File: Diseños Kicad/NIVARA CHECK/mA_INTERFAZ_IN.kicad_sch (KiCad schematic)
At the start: 1 part

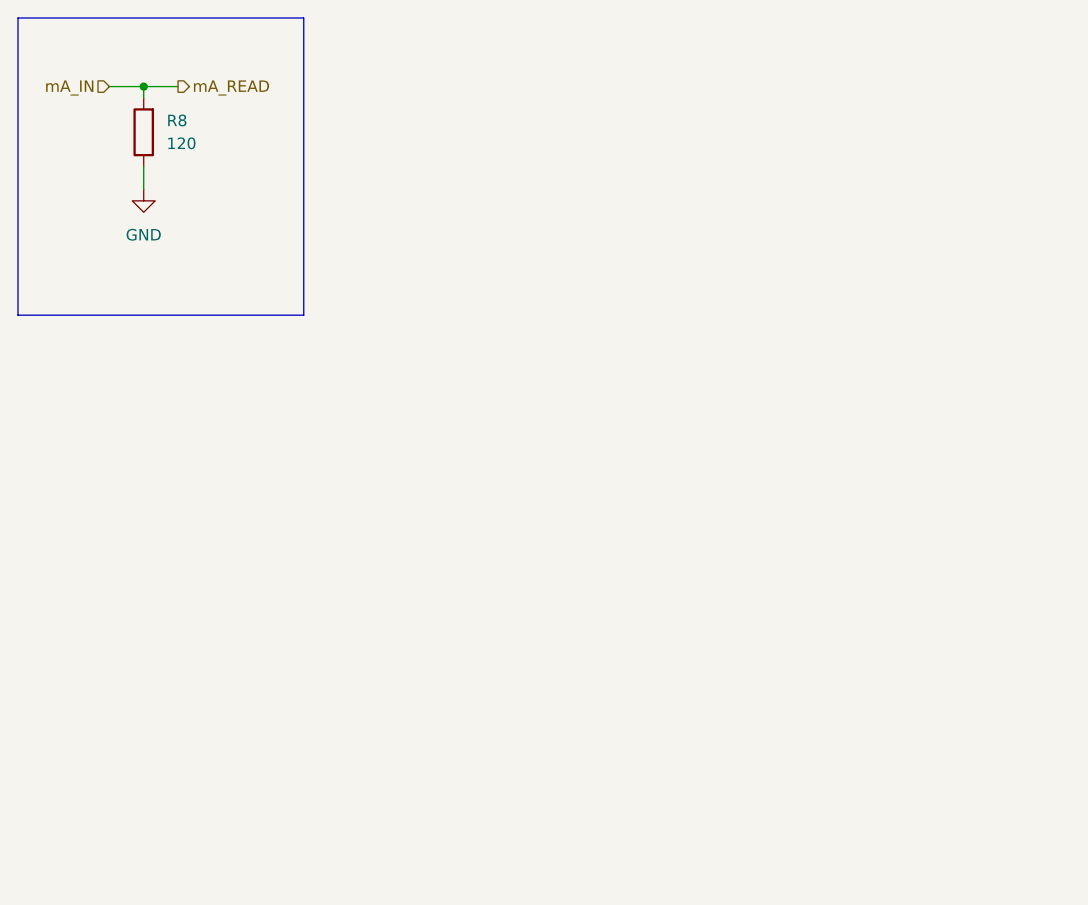
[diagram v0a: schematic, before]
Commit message: ACTUALIZACION HECHA
PCB SUPUESTA
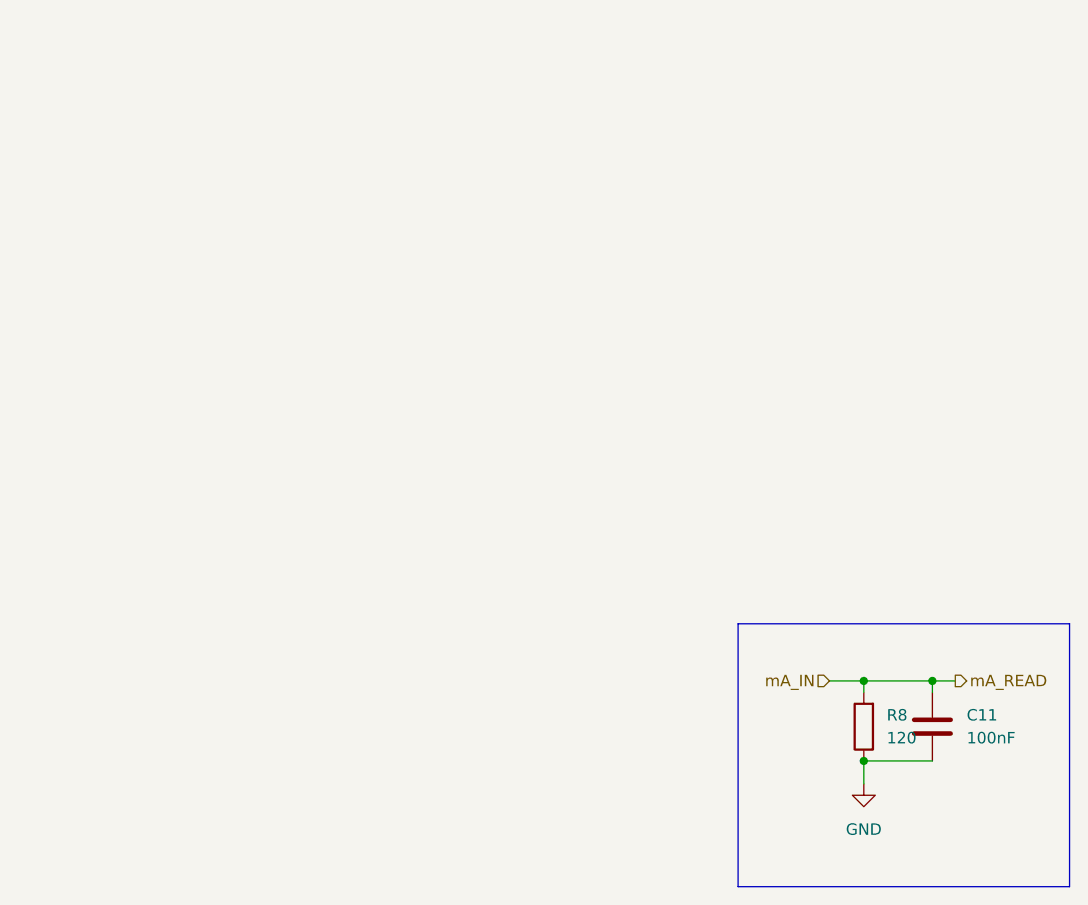
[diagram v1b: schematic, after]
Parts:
- added C11: 100nF, symbol Device:C
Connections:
- net GND: now also C11.2
- net mA_IN: now also C11.1
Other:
- moved on the sheet: R8
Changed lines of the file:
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@@
 	(paper "A4")
 	(rectangle
-		(start 20.32 17.78)
-		(end 52.07 50.8)
+		(start 100.33 85.09)
+		(end 137.16 114.3)
 		(stroke
 			(width 0)
@@
 	)
 	(junction
-		(at 34.29 25.4)
+		(at 114.3 100.33)
 		(diameter 0)
 		(color 0 0 0 0)
 	)
-	(wire
-		(pts
-			(xy 34.29 25.4) (xy 34.29 26.67)
-		)
-		(stroke
-			(width 0)
-			(type default)
-		)
-	)
-	(wire
-		(pts
-			(xy 30.48 25.4) (xy 34.29 25.4)
-		)
-		(stroke
-			(width 0)
-			(type default)
-		)
-	)
-	(wire
-		(pts
-			(xy 34.29 25.4) (xy 38.1 25.4)
-		)
-		(stroke
-			(width 0)
-			(type default)
-		)
-	)
-	(wire
-		(pts
-			(xy 34.29 34.29) (xy 34.29 36.83)
+	(junction
+		(at 114.3 91.44)
+		(diameter 0)
+		(color 0 0 0 0)
+	)
+	(junction
+		(at 121.92 91.44)
+		(diameter 0)
+		(color 0 0 0 0)
+	)
+	(wire
+		(pts
+			(xy 114.3 91.44) (xy 114.3 92.71)
+		)
+		(stroke
+			(width 0)
+			(type default)
+		)
+	)
+	(wire
+		(pts
+			(xy 121.92 91.44) (xy 124.46 91.44)
+		)
+		(stroke
+			(width 0)
+			(type default)
+		)
+	)
+	(wire
+		(pts
+			(xy 110.49 91.44) (xy 114.3 91.44)
+		)
+		(stroke
+			(width 0)
+			(type default)
+		)
+	)
+	(wire
+		(pts
+			(xy 114.3 100.33) (xy 121.92 100.33)
+		)
+		(stroke
+			(width 0)
+			(type default)
+		)
+	)
+	(wire
+		(pts
+			(xy 121.92 91.44) (xy 121.92 92.71)
+		)
+		(stroke
+			(width 0)
+			(type default)
+		)
+	)
+	(wire
+		(pts
+			(xy 114.3 91.44) (xy 121.92 91.44)
+		)
+		(stroke
+			(width 0)
+			(type default)
+		)
+	)
+	(wire
+		(pts
+			(xy 114.3 100.33) (xy 114.3 102.87)
 		)
 		(stroke
@@
 	(hierarchical_label "mA_IN"
 		(shape input)
-		(at 30.48 25.4 180)
+		(at 110.49 91.44 180)
 		(effects
 			(font
@@
 	(hierarchical_label "mA_READ"
 		(shape output)
-		(at 38.1 25.4 0)
+		(at 124.46 91.44 0)
 		(effects
 			(font
@@
 	(symbol
 		(lib_id "Device:R")
-		(at 34.29 30.48 180)
+		(at 114.3 96.52 180)
 		(unit 1)
 		(exclude_from_sim no)
@@
 		(fields_autoplaced yes)
 		(property "Reference" "R8"
-			(at 36.83 29.2099 0)
+			(at 116.84 95.2499 0)
 			(effects
 				(font
@@
 		)
 		(property "Value" "120"
-			(at 36.83 31.7499 0)
+			(at 116.84 97.7899 0)
 			(effects
 				(font
@@
 		)
 		(property "Footprint" ""
-			(at 36.068 30.48 90)
+			(at 116.078 96.52 90)
 			(effects
 				(font
@@
 		)
 		(property "Datasheet" "~"
-			(at 34.29 30.48 0)
+			(at 114.3 96.52 0)
 			(effects
 				(font
@@
 		)
 		(property "Description" "Resistor"
-			(at 34.29 30.48 0)
+			(at 114.3 96.52 0)
 			(effects
 				(font
@@
 		)
 		(property "Tolerance" "0.1-1%"
-			(at 34.29 30.48 0)
+			(at 114.3 96.52 0)
 			(effects
 				(font
@@
 		)
 		(instances
-			(project ""
+			(project "NIVARA"
 				(path "/8290cc18-06d0-4e02-a781-29a61ebc321a/9e4d7a0c-a5eb-4e88-9036-0c35e68b279a/89d29688-da71-49bb-a25b-d6f160f4d0d4"
 					(reference "R8")
@@
 	)
 	(symbol
+		(lib_id "Device:C")
+		(at 121.92 96.52 0)
+		(unit 1)
+		(exclude_from_sim no)
+		(in_bom yes)
+		(on_board yes)
+		(dnp no)
+		(fields_autoplaced yes)
+		(property "Reference" "C11"
+			(at 125.73 95.2499 0)
+			(effects
+				(font
+					(size 1.27 1.27)
+				)
+				(justify left)
+			)
+		)
+		(property "Value" "100nF"
+			(at 125.73 97.7899 0)
+			(effects
+				(font
+					(size 1.27 1.27)
+				)
+				(justify left)
+			)
+		)
+		(property "Footprint" ""
+			(at 122.8852 100.33 0)
+			(effects
+				(font
+					(size 1.27 1.27)
+				)
+				(hide yes)
+			)
+		)
+		(property "Datasheet" "~"
+			(at 121.92 96.52 0)
+			(effects
+				(font
+					(size 1.27 1.27)
+				)
+				(hide yes)
+			)
+		)
+		(property "Description" "Unpolarized capacitor"
+			(at 121.92 96.52 0)
+			(effects
+				(font
+					(size 1.27 1.27)
+				)
+				(hide yes)
+			)
+		)
+		(pin "2"
+		)
+		(pin "1"
+		)
+		(instances
+			(project "NIVARA"
+				(path "/8290cc18-06d0-4e02-a781-29a61ebc321a/9e4d7a0c-a5eb-4e88-9036-0c35e68b279a/89d29688-da71-49bb-a25b-d6f160f4d0d4"
+					(reference "C11")
+					(unit 1)
+				)
+			)
+		)
+	)
+	(symbol
 		(lib_id "power:GND")
-		(at 34.29 36.83 0)
+		(at 114.3 102.87 0)
 		(unit 1)
 		(exclude_from_sim no)
@@
 		(fields_autoplaced yes)
 		(property "Reference" "#PWR029"
-			(at 34.29 43.18 0)
+			(at 114.3 109.22 0)
 			(effects
 				(font
@@
 		)
 		(property "Value" "GND"
-			(at 34.29 41.91 0)
+			(at 114.3 107.95 0)
 			(effects
 				(font
@@
 		)
 		(property "Footprint" ""
-			(at 34.29 36.83 0)
+			(at 114.3 102.87 0)
 			(effects
 				(font
@@
 		)
 		(property "Datasheet" ""
-			(at 34.29 36.83 0)
+			(at 114.3 102.87 0)
 			(effects
 				(font
@@
 		)
 		(property "Description" "Power symbol creates a global label with name \"GND\" , ground"
-			(at 34.29 36.83 0)
+			(at 114.3 102.87 0)
 			(effects
 				(font
@@
 		)
 		(instances
-			(project ""
+			(project "NIVARA"
 				(path "/8290cc18-06d0-4e02-a781-29a61ebc321a/9e4d7a0c-a5eb-4e88-9036-0c35e68b279a/89d29688-da71-49bb-a25b-d6f160f4d0d4"
 					(reference "#PWR029")
